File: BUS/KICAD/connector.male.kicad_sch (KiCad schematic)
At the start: 1 part, among them J2 Conn_02x20_Odd_Even

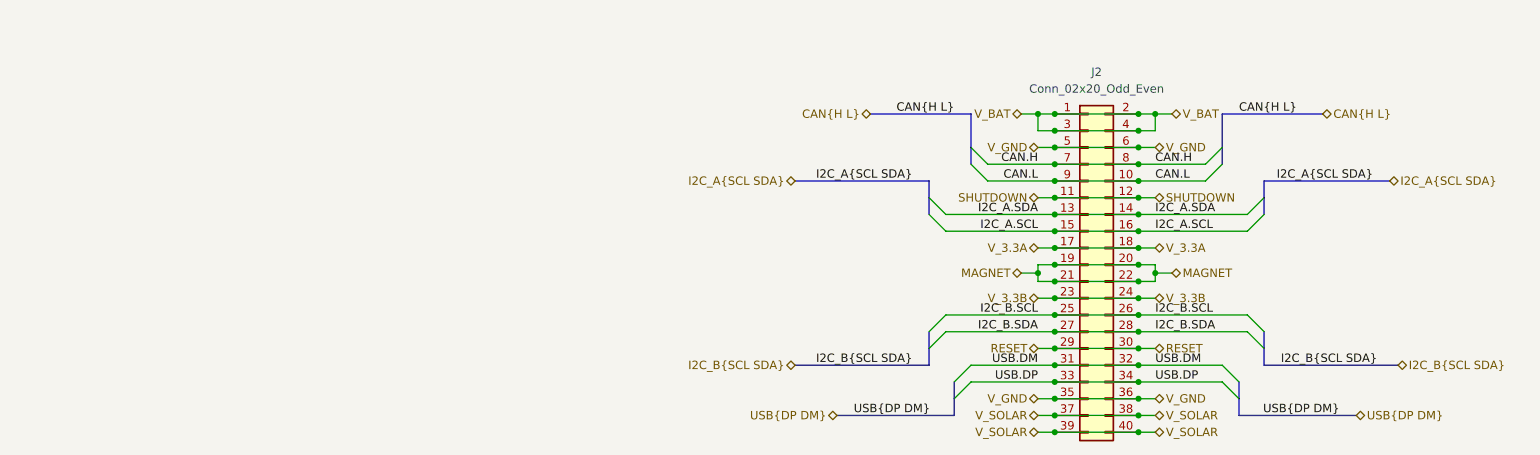
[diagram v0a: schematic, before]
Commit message: Updated Bus
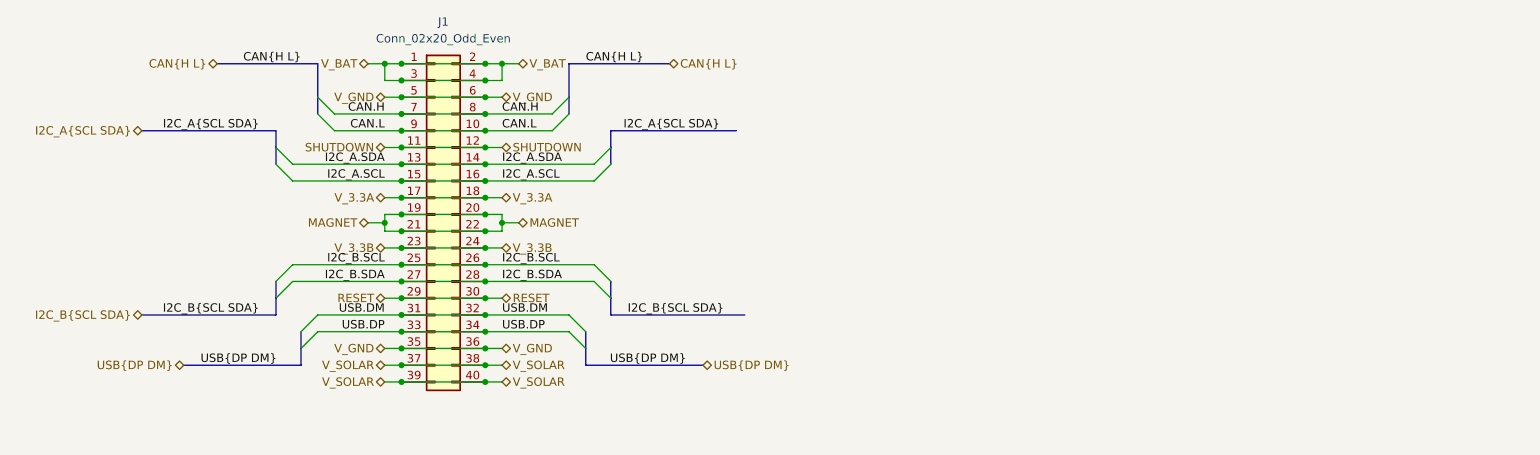
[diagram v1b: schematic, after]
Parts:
- removed J2: Conn_02x20_Odd_Even, Connector_PinHeader_2.00mm:PinHeader_2x20_P2.00mm_Horizontal, symbol Connector_Generic:Conn_02x20_Odd_Even
- added J1: Conn_02x20_Odd_Even, Connector_PinHeader_2.00mm:PinHeader_2x20_P2.00mm_Horizontal, symbol Connector_Generic:Conn_02x20_Odd_Even
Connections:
- net CAN.H: now also J1.7 (Pin_7), J1.8 (Pin_8)
- net CAN.L: now also J1.10 (Pin_10), J1.9 (Pin_9)
- net I2C_A.SCL: now also J1.15 (Pin_15), J1.16 (Pin_16)
- net I2C_A.SDA: now also J1.13 (Pin_13), J1.14 (Pin_14)
- net I2C_B.SCL: now also J1.25 (Pin_25), J1.26 (Pin_26)
- net I2C_B.SDA: now also J1.27 (Pin_27), J1.28 (Pin_28)
- net MAGNET: now also J1.19 (Pin_19), J1.20 (Pin_20), J1.21 (Pin_21), J1.22 (Pin_22)
- net RESET: now also J1.29 (Pin_29), J1.30 (Pin_30)
- net SHUTDOWN: now also J1.11 (Pin_11), J1.12 (Pin_12)
- net USB.DM: now also J1.31 (Pin_31), J1.32 (Pin_32)
- net USB.DP: now also J1.33 (Pin_33), J1.34 (Pin_34)
- net V_3.3A: now also J1.17 (Pin_17), J1.18 (Pin_18)
- net V_3.3B: now also J1.23 (Pin_23), J1.24 (Pin_24)
- net V_BAT: now also J1.1 (Pin_1), J1.2 (Pin_2), J1.3 (Pin_3), J1.4 (Pin_4)
- net V_GND: now also J1.35 (Pin_35), J1.36 (Pin_36), J1.5 (Pin_5), J1.6 (Pin_6)
- net V_SOLAR: now also J1.37 (Pin_37), J1.38 (Pin_38), J1.39 (Pin_39), J1.40 (Pin_40)
